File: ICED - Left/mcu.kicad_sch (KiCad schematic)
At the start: 48 parts, among them P1 Conn_ARM_JTAG_SWD_10, P2 DX07S024XJ1R1100, P3 CONN_17, P4 692121130100, P5 RGB Out, Q1 TC1264, U1 MK20DX256VLH7, X1 NX3225SA-16.000MHZ-STD-CSR-

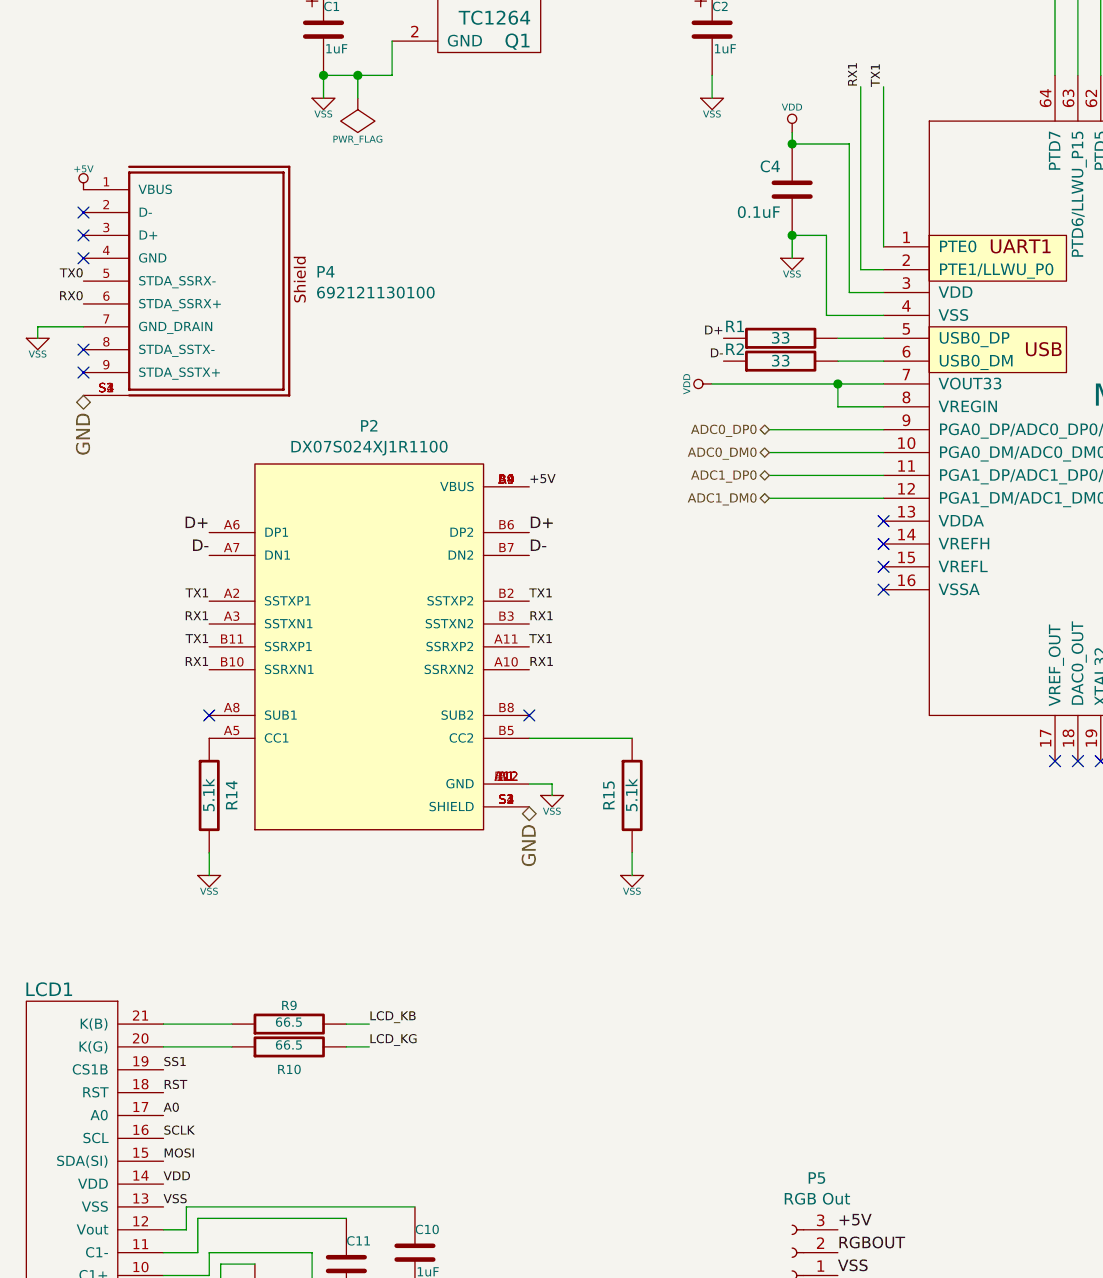
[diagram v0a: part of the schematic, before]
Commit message: More routing
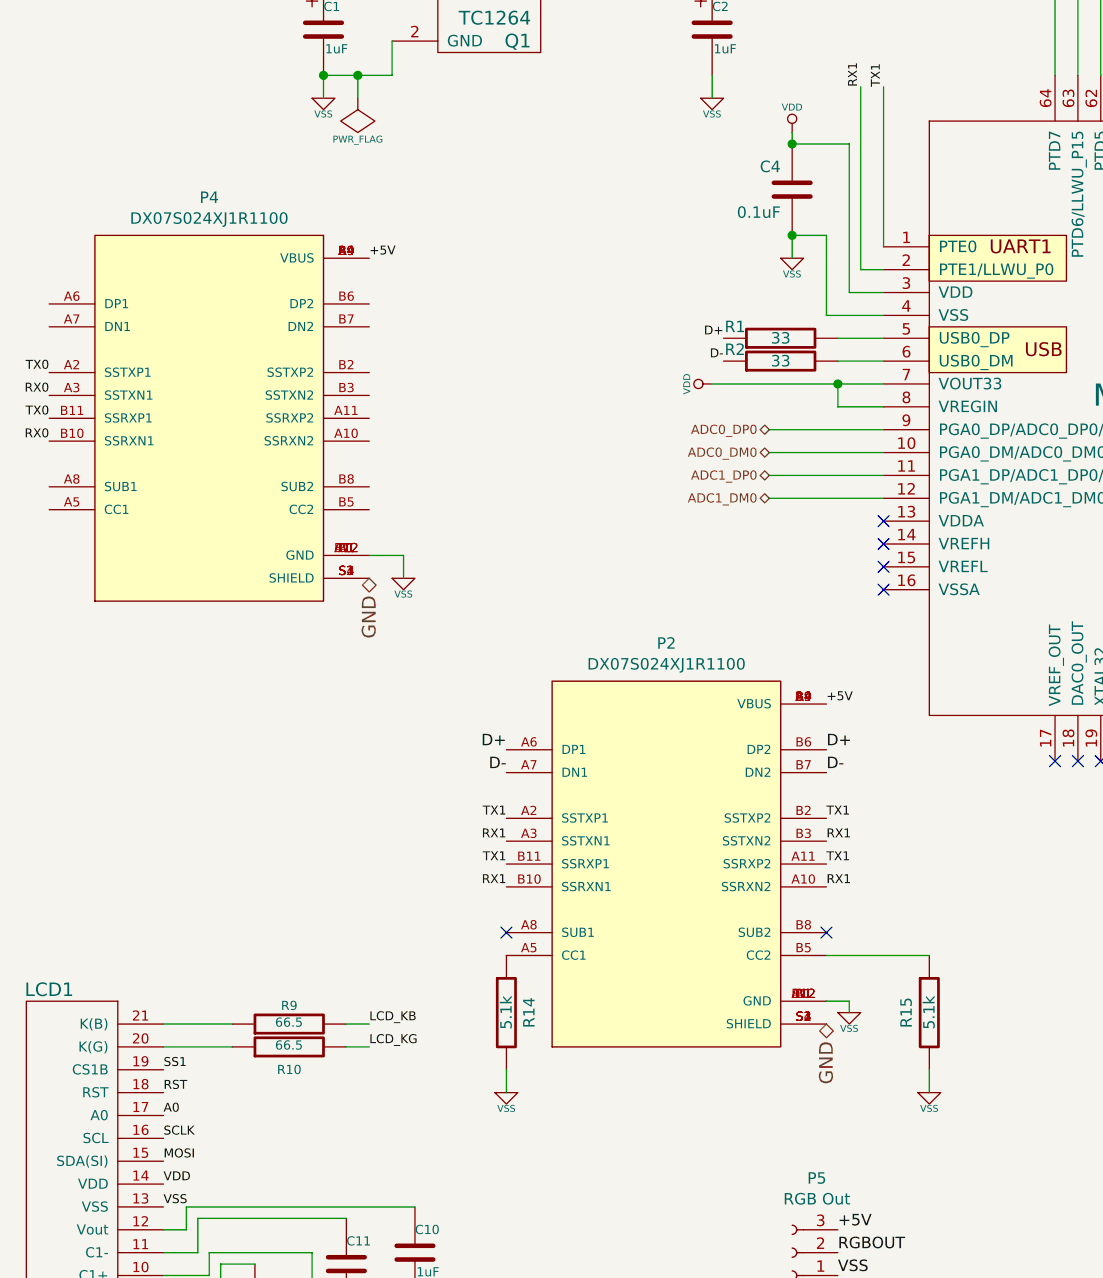
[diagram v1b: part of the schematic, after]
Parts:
- removed P4: 692121130100, 692121130100, symbol ICEDLeft:692121130100
- added P4: DX07S024XJ1R1100, JAE_DX07S024XJ1R1100, symbol ICEDLeft:DX07S024XJ1R1100
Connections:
- net +5V: now also P4.A4 (VBUS), P4.A9 (VBUS), P4.B4 (VBUS), P4.B9 (VBUS)
- net GND: now also P4.S1 (SHIELD), P4.S2 (SHIELD), P4.S3 (SHIELD), P4.S4 (SHIELD)
- net RX0: now also P4.A3 (SSTXN1), P4.B10 (SSRXN1)
- net TX0: now also P4.A2 (SSTXP1), P4.B11 (SSRXP1)
- net VSS: now also P4.A1 (GND), P4.A12 (GND), P4.B1 (GND), P4.B12 (GND)
- no-connect marks 18 -> 13
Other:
- moved on the sheet: P2, R14, R15
